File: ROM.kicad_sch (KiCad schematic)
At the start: 6 parts, among them U19 SN74ALS04 (КР1533ЛН1), U70 27C64, U71 27C64, U75 IN74ALS32N (КР1533ЛЛ1), U76 27C256

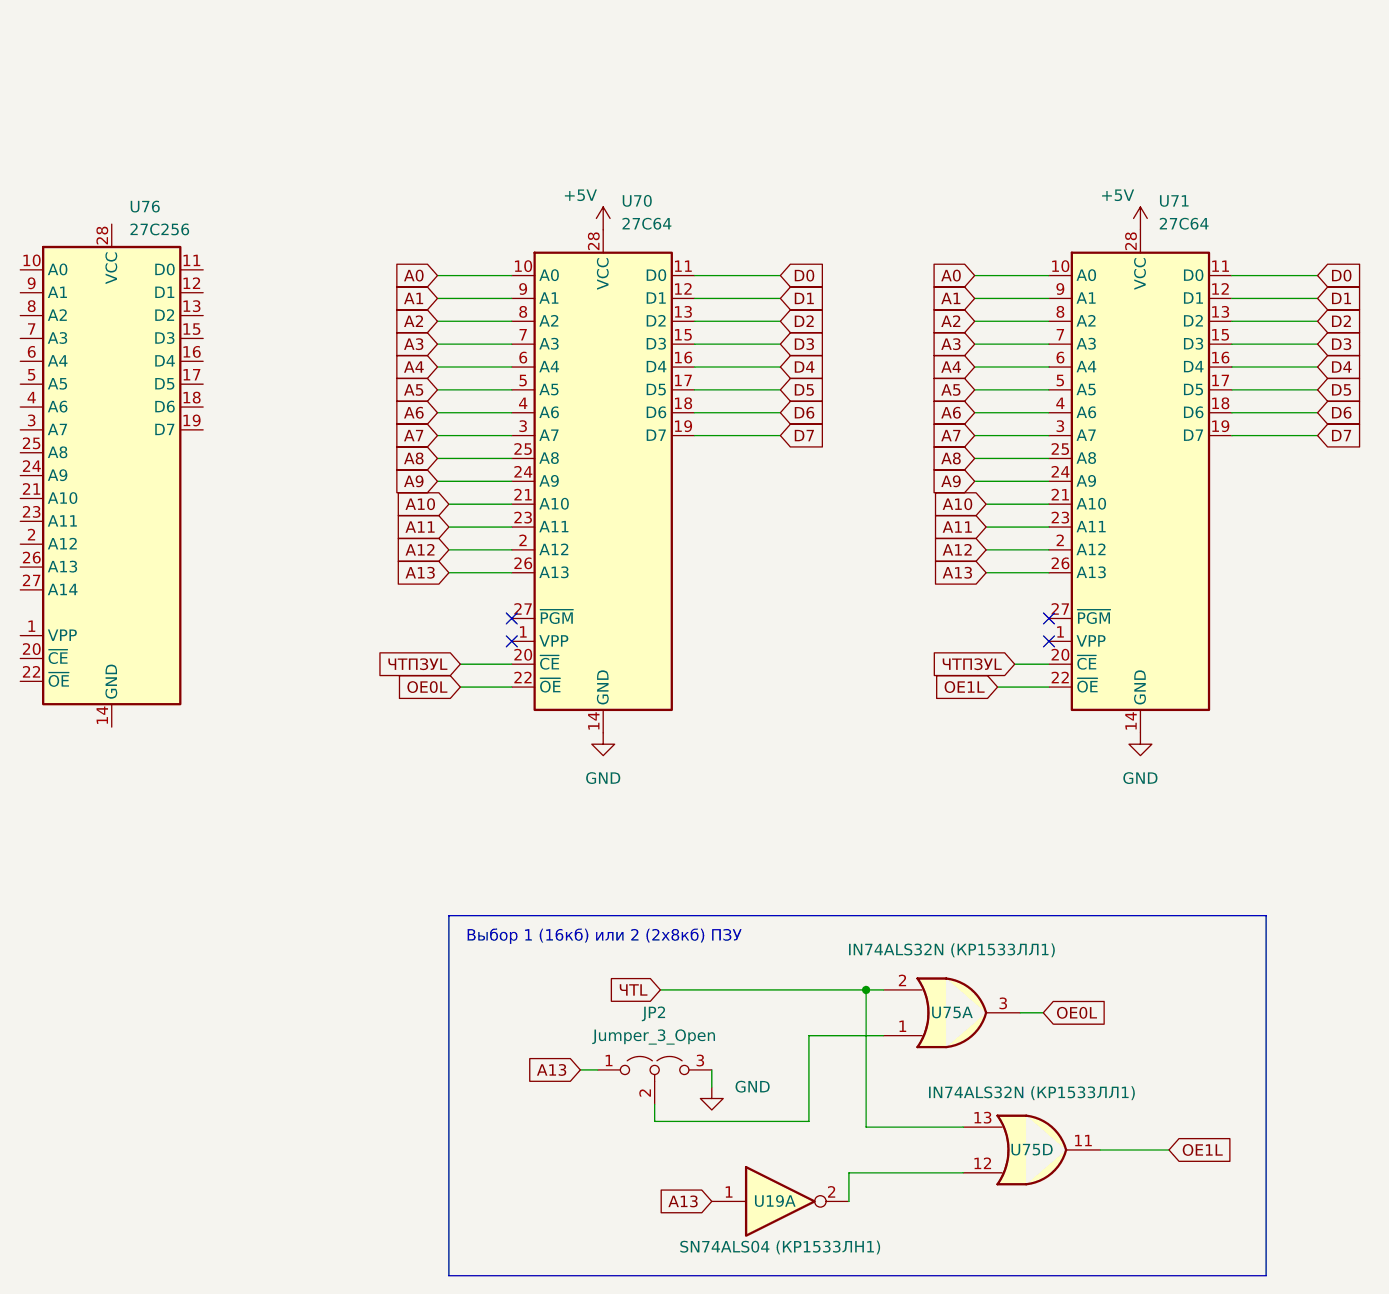
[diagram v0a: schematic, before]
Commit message: Topology for version 1.2
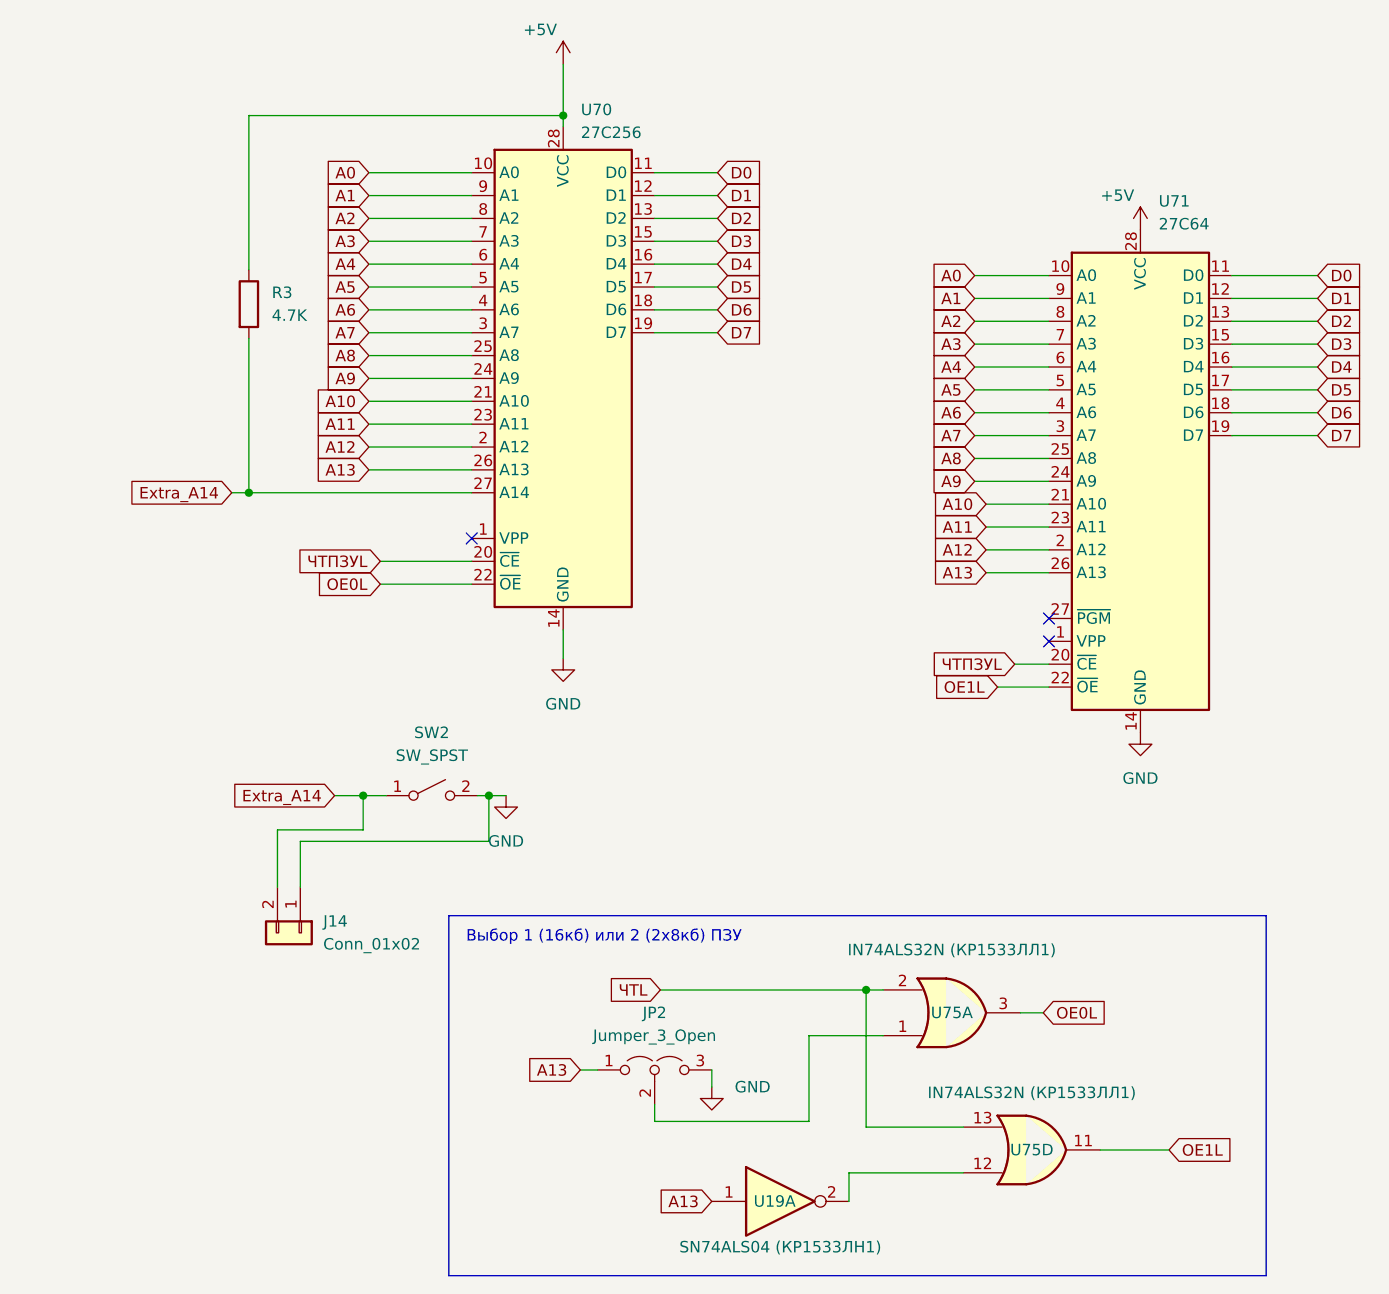
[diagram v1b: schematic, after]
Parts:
- removed U70: 27C64, Delta_sm_lib:DIP-28_W15.24mm_Socket, symbol Delta_s_m_Lib:27C128
- added J14: Conn_01x02, Connector_PinHeader_2.54mm:PinHeader_1x02_P2.54mm_Vertical, symbol Connector_Generic:Conn_01x02
- added R3: 4.7K, Delta_sm_lib:R_Axial_DIN0207_L6.3mm_D2.5mm_P10.16mm_Horizontal, symbol Delta_s_m_Lib:R
- added SW2: SW_SPST, Delta_sm_lib:onoffswitch, symbol Switch:SW_SPST
- renumbered U76 to U70
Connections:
- net +5V: now also U70.28 (VCC), R3.1
- net A0: now also U70.10 (A0)
- net A1: now also U70.9 (A1)
- net A10: now also U70.21 (A10)
- net A11: now also U70.23 (A11)
- net A12: now also U70.2 (A12)
- net A13: now also U70.26 (A13)
- net A2: now also U70.8 (A2)
- net A3: now also U70.7 (A3)
- net A4: now also U70.6 (A4)
- net A5: now also U70.5 (A5)
- net A6: now also U70.4 (A6)
- net A7: now also U70.3 (A7)
- net A8: now also U70.25 (A8)
- net A9: now also U70.24 (A9)
- net D0: now also U70.11 (D0)
- net D1: now also U70.12 (D1)
- net D2: now also U70.13 (D2)
- net D3: now also U70.15 (D3)
- net D4: now also U70.16 (D4)
- net D5: now also U70.17 (D5)
- net D6: now also U70.18 (D6)
- net D7: now also U70.19 (D7)
- net GND: now also U70.14 (GND), J14.1 (Pin_1), SW2.2 (B)
- net OE0L: now also U70.22 (~{OE})
- net ЧТПЗУL: now also U70.20 (~{CE})
- net Extra_A14: now reaches U70.27 (A14)
- net Extra_A14: now also J14.2 (Pin_2), R3.2, SW2.1 (A)
- no-connect marks 4 -> 3
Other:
- moved on the sheet: U70
